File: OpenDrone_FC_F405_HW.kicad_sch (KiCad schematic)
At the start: 83 parts, among them J1 Conn_01x05, J10 Conn_01x02, J11 Conn_01x05, J12 Conn_01x05, J13 Conn_01x02, J14 Conn_01x02, J15 Conn_02x04_Odd_Even, J16 Conn_01x05, J2 Conn_01x02, J3 Conn_01x02, J4 Conn_01x02, J5 Conn_01x02, J6 Conn_01x08, J7 Conn_01x02, J8 Conn_01x04, J9 Conn_01x02, U1 STM32F405RGTx, U2 TPS5430DDA, U3 TPS5430DDA, U4 MPU6000, U5 HMC5883L, U6 BMP280, U8 Board, Y1 8MHz

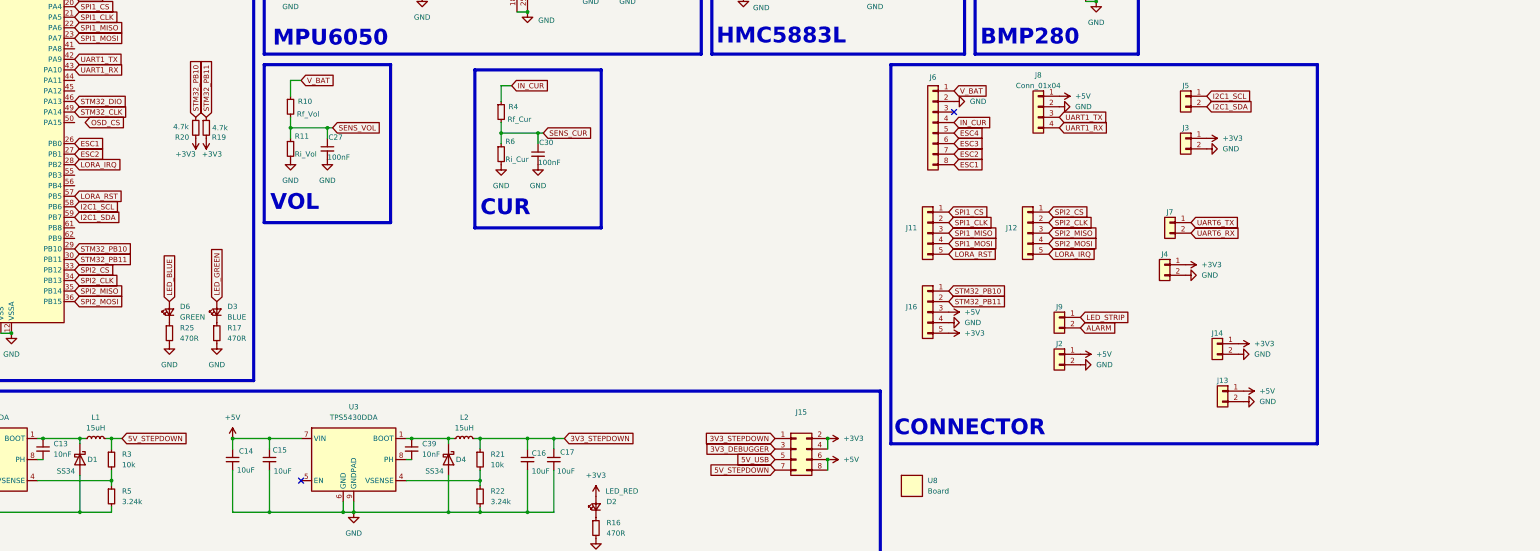
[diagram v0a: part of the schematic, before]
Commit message: update project
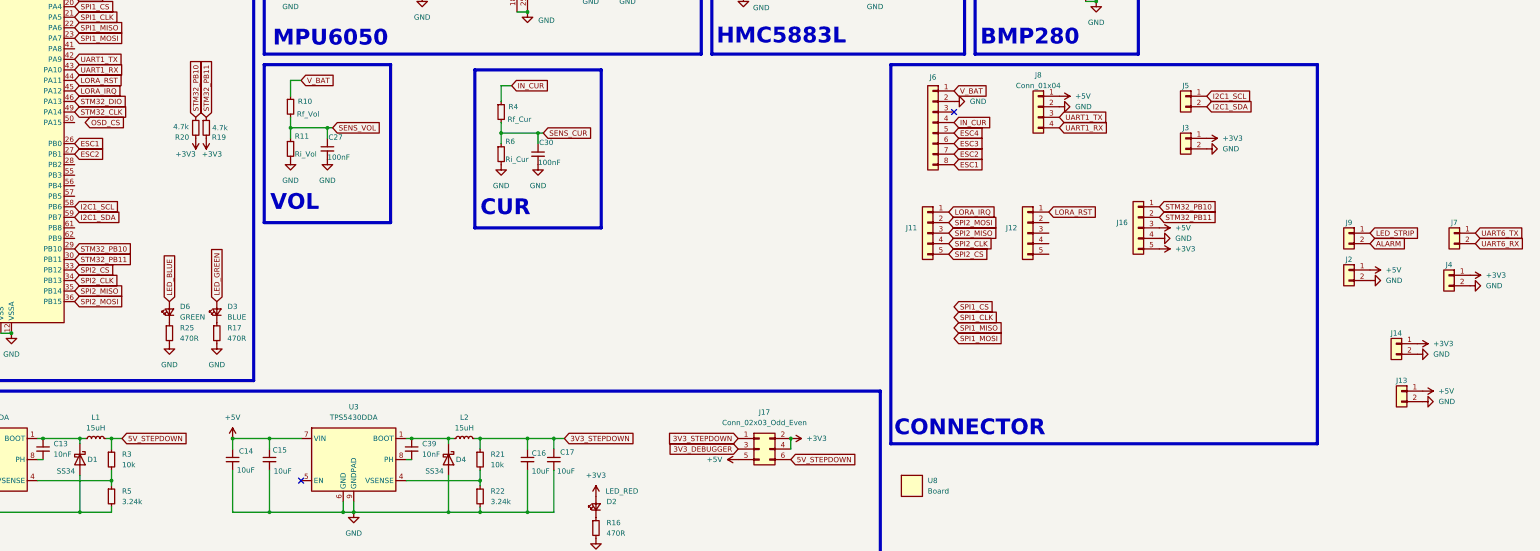
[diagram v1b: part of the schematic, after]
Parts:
- removed J15: Conn_02x04_Odd_Even, Connector_PinHeader_1.27mm:PinHeader_2x04_P1.27mm_Vertical, symbol Connector_Generic:Conn_02x04_Odd_Even
- added J17: Conn_02x03_Odd_Even, Connector_PinHeader_1.27mm:PinHeader_2x03_P1.27mm_Vertical, symbol Connector_Generic:Conn_02x03_Odd_Even
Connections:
- net +3V3: now also J17.2 (Pin_2), J17.4 (Pin_4)
- net +5V: now also J17.5 (Pin_5)
- net 3V3_DEBUGGER: now also J17.3 (Pin_3)
- net 3V3_STEPDOWN: now also J17.1 (Pin_1)
- net 5V_STEPDOWN: now also J17.6 (Pin_6)
- net LORA_IRQ: now also J11.1 (Pin_1), U1.45 (PA12); no longer J12.5 (Pin_5), U1.28 (PB2)
- net LORA_RST: now also J12.1 (Pin_1), U1.44 (PA11); no longer J11.5 (Pin_5), U1.57 (PB5)
- net SPI1_CLK: no longer J11.2 (Pin_2)
- net SPI1_CS: no longer J11.1 (Pin_1)
- net SPI1_MISO: no longer J11.3 (Pin_3)
- net SPI1_MOSI: no longer J11.4 (Pin_4)
- net SPI2_CLK: now also J11.4 (Pin_4); no longer J12.2 (Pin_2)
- net SPI2_CS: now also J11.5 (Pin_5); no longer J12.1 (Pin_1)
- net SPI2_MISO: now also J11.3 (Pin_3); no longer J12.3 (Pin_3)
- net SPI2_MOSI: now also J11.2 (Pin_2); no longer J12.4 (Pin_4)
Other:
- moved on the sheet: J13, J14, J16, J2, J4, J7, J9

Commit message: update project
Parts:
- removed J10: Conn_01x02, Footprint:MountingPad_Battery, symbol Connector_Generic:Conn_01x02
- removed R19, R20: 4.7k, Resistor_SMD:R_0402_1005Metric, symbol Device:R_Small
- added C34: 100nF, Capacitor_SMD:C_0402_1005Metric, symbol Device:C_Small
- added SW1: RESET, Footprint:Button_SMD_4.2x3.3x2.5mm, symbol Switch:SW_Push
- C15: footprint Capacitor_SMD:C_1210_3225Metric -> Capacitor_SMD:C_1206_3216Metric
- J11, J12, J16: footprint Connector_PinHeader_2.00mm:PinHeader_1x05_P2.00mm_Vertical -> Footprint:Header_1x05_P2.00mm_Vertical
- J17: footprint Connector_PinHeader_1.27mm:PinHeader_2x03_P1.27mm_Vertical -> Connector_PinHeader_2.00mm:PinHeader_2x03_P2.00mm_Vertical
- L1, L2: footprint Footprint:Inductor_SMD_5D28 -> Footprint:Inductor_SMD_4D28
- U6: footprint Package_LGA:Bosch_LGA-8_2x2.5mm_P0.65mm_ClockwisePinNumbering -> Footprint:LGA-8_2x2.5mm_P0.65mm
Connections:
- net +3V3: now also J11.5 (Pin_5); no longer J14.1 (Pin_1), J16.5 (Pin_5), J3.1 (Pin_1), J4.1 (Pin_1)
- net +5V: now also J16.5 (Pin_5), J3.1 (Pin_1), J4.1 (Pin_1); no longer J16.3 (Pin_3)
- net 3V3_DEBUGGER: now also J17.1 (Pin_1); no longer J17.3 (Pin_3)
- net 3V3_STEPDOWN: now also J17.3 (Pin_3); no longer J17.1 (Pin_1)
- net ESC1: now also U1.16 (PA2); no longer U1.26 (PB0)
- net ESC2: now also U1.17 (PA3); no longer U1.27 (PB1)
- net ESC3: now also U1.26 (PB0); no longer U1.17 (PA3)
- net ESC4: now also U1.27 (PB1); no longer U1.16 (PA2)
- net GND: now also J1.2 (Pin_2), J12.5 (Pin_5), C34.2, SW1.1; no longer J1.5 (Pin_5), J14.2 (Pin_2), J16.4 (Pin_4)
- net I2C1_SCL: now also J12.4 (Pin_4); no longer J5.1 (Pin_1), R8.2, U4.23 (SCL/SCLK), U6.4 (SCK)
- net I2C1_SDA: now also J12.3 (Pin_3); no longer J5.2 (Pin_2), R7.2, U4.24 (SDA/SDI), U6.3 (SDI)
- net LED_BLUE: now also U1.40 (PC9); no longer U1.3 (PC14)
- net LED_GREEN: now also U1.39 (PC8); no longer U1.2 (PC13)
- net LORA_IRQ: now also J12.2 (Pin_2); no longer J11.1 (Pin_1)
- net MPU6000_INT: now also U1.11 (PC3); no longer U1.15 (PA1)
- net SPI1_CLK: now also J16.2 (Pin_2)
- net SPI1_CS: now also J16.1 (Pin_1)
- net SPI1_MISO: now also J16.3 (Pin_3)
- net SPI1_MOSI: now also J16.4 (Pin_4)
- net SPI2_CLK: now also J11.3 (Pin_3); no longer J11.4 (Pin_4)
- net SPI2_CS: now also J11.4 (Pin_4); no longer J11.5 (Pin_5)
- net SPI2_MISO: now also J11.2 (Pin_2); no longer J11.3 (Pin_3)
- net SPI2_MOSI: now also J11.1 (Pin_1); no longer J11.2 (Pin_2)
- net STM32_CLK: now also J1.4 (Pin_4); no longer J1.3 (Pin_3)
- net STM32_DIO: now also J1.5 (Pin_5); no longer J1.2 (Pin_2)
- net STM32_NRST: now also J1.3 (Pin_3), C34.1, SW1.2; no longer J1.4 (Pin_4)
- net UART4_TX: now reaches U1.14 (PA0)
- net UART4_TX: now also J14.1 (Pin_1)
- net LED_STRIP2: now reaches U1.61 (PB8)
- net LED_STRIP2: now also J9.2 (Pin_2)
- net LED_STRIP1: now reaches U1.62 (PB9)
- net LED_STRIP1: now also J9.1 (Pin_1)
- net ALARM: no longer names the net of U1.8 (PC0)
- net ALARM: no longer J9.2 (Pin_2)
- net LED_STRIP: no longer names the net of U1.4 (PC15)
- net LED_STRIP: no longer J9.1 (Pin_1)
- net STM32_PB10 renamed I2C2_SCL
- net I2C2_SCL: now also J5.1 (Pin_1), R8.2, U4.23 (SCL/SCLK), U6.4 (SCK); no longer J16.1 (Pin_1)
- net STM32_PB11 renamed I2C2_SDA
- net I2C2_SDA: now also J5.2 (Pin_2), R7.2, U4.24 (SDA/SDI), U6.3 (SDI); no longer J16.2 (Pin_2)
- new net UART4_RX: J14.2 (Pin_2), U1.15 (PA1)
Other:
- moved on the sheet: J14, R1

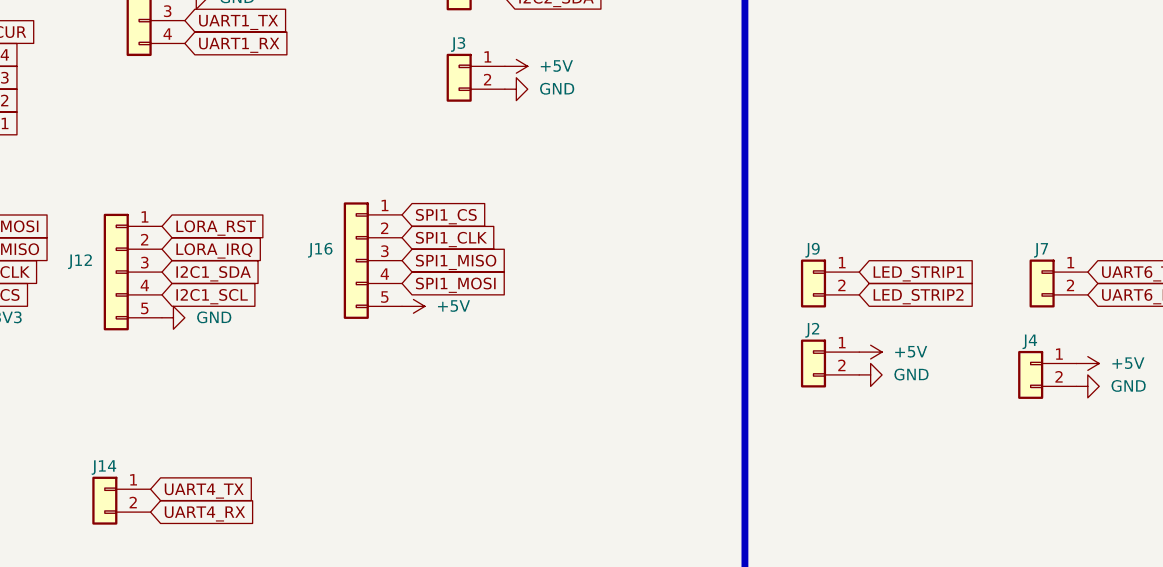
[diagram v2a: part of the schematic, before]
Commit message: update project
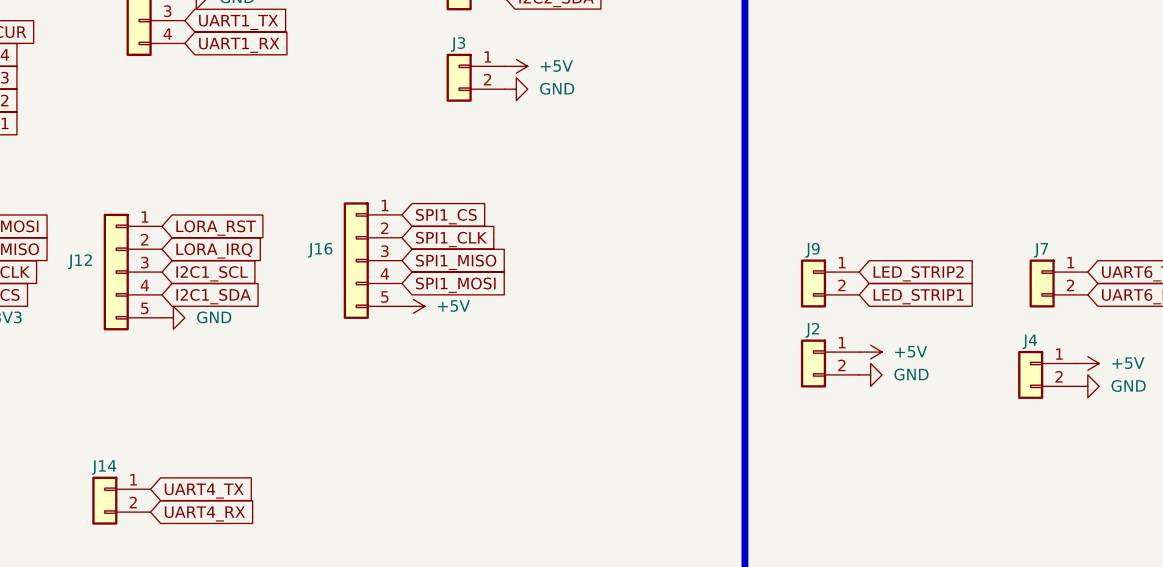
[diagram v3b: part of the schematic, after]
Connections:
- net I2C1_SCL: now also J12.3 (Pin_3); no longer J12.4 (Pin_4)
- net I2C1_SDA: now also J12.4 (Pin_4); no longer J12.3 (Pin_3)
- net LED_STRIP1: now also J9.2 (Pin_2); no longer J9.1 (Pin_1)
- net LED_STRIP2: now also J9.1 (Pin_1); no longer J9.2 (Pin_2)
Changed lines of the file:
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@@
 	(global_label "LED_STRIP1"
 		(shape input)
+		(at 396.24 115.57 0)
+		(fields_autoplaced yes)
+		(effects
+			(font
+				(size 1.27 1.27)
+			)
+			(justify left)
+		)
+		(property "Intersheetrefs" "${INTERSHEET_REFS}"
+			(at 410.1713 115.57 0)
+			(effects
+				(font
+					(size 1.27 1.27)
+				)
+				(justify left)
+				(hide yes)
+			)
+		)
+	)
+	(global_label "I2C1_SDA"
+		(shape input)
+		(at 318.77 115.57 0)
+		(fields_autoplaced yes)
+		(effects
+			(font
+				(size 1.27 1.27)
+			)
+			(justify left)
+		)
+		(property "Intersheetrefs" "${INTERSHEET_REFS}"
+			(at 330.5847 115.57 0)
+			(effects
+				(font
+					(size 1.27 1.27)
+				)
+				(justify left)
+				(hide yes)
+			)
+		)
+	)
+	(global_label "STM32_NRST"
+		(shape input)
+		(at 48.26 48.26 180)
+		(fields_autoplaced yes)
+		(effects
+			(font
+				(size 1.27 1.27)
+			)
+			(justify right)
+		)
+		(property "Intersheetrefs" "${INTERSHEET_REFS}"
+			(at 33.4821 48.26 0)
+			(effects
+				(font
+					(size 1.27 1.27)
+				)
+				(justify right)
+				(hide yes)
+			)
+		)
+	)
+	(global_label "I2C1_SCL"
+		(shape input)
+		(at 318.77 113.03 0)
+		(fields_autoplaced yes)
+		(effects
+			(font
+				(size 1.27 1.27)
+			)
+			(justify left)
+		)
+		(property "Intersheetrefs" "${INTERSHEET_REFS}"
+			(at 330.5242 113.03 0)
+			(effects
+				(font
+					(size 1.27 1.27)
+				)
+				(justify left)
+				(hide yes)
+			)
+		)
+	)
+	(global_label "I2C2_SCL"
+		(shape input)
+		(at 151.13 29.21 180)
+		(fields_autoplaced yes)
+		(effects
+			(font
+				(size 1.27 1.27)
+			)
+			(justify right)
+		)
+		(property "Intersheetrefs" "${INTERSHEET_REFS}"
+			(at 139.3758 29.21 0)
+			(effects
+				(font
+					(size 1.27 1.27)
+				)
+				(justify right)
+				(hide yes)
+			)
+		)
+	)
+	(global_label "UART4_RX"
+		(shape input)
+		(at 83.82 50.8 0)
+		(fields_autoplaced yes)
+		(effects
+			(font
+				(size 1.27 1.27)
+			)
+			(justify left)
+		)
+		(property "Intersheetrefs" "${INTERSHEET_REFS}"
+			(at 96.1185 50.8 0)
+			(effects
+				(font
+					(size 1.27 1.27)
+				)
+				(justify left)
+				(hide yes)
+			)
+		)
+	)
+	(global_label "LED_STRIP2"
+		(shape input)
+		(at 83.82 111.76 0)
+		(fields_autoplaced yes)
+		(effects
+			(font
+				(size 1.27 1.27)
+			)
+			(justify left)
+		)
+		(property "Intersheetrefs" "${INTERSHEET_REFS}"
+			(at 97.7513 111.76 0)
+			(effects
+				(font
+					(size 1.27 1.27)
+				)
+				(justify left)
+				(hide yes)
+			)
+		)
+	)
+	(global_label "5V_STEPDOWN"
+		(shape input)
+		(at 256.54 167.64 0)
+		(fields_autoplaced yes)
+		(effects
+			(font
+				(size 1.27 1.27)
+			)
+			(justify left)
+		)
+		(property "Intersheetrefs" "${INTERSHEET_REFS}"
+			(at 272.7694 167.64 0)
+			(effects
+				(font
+					(size 1.27 1.27)
+				)
+				(justify left)
+				(hide yes)
+			)
+		)
+	)
+	(global_label "IN_CUR"
+		(shape input)
+		(at 189.23 77.47 0)
+		(fields_autoplaced yes)
+		(effects
+			(font
+				(size 1.27 1.27)
+			)
+			(justify left)
+		)
+		(property "Intersheetrefs" "${INTERSHEET_REFS}"
+			(at 198.9886 77.47 0)
+			(effects
+				(font
+					(size 1.27 1.27)
+				)
+				(justify left)
+				(hide yes)
+			)
+		)
+	)
+	(global_label "LED_STRIP2"
+		(shape input)
 		(at 396.24 113.03 0)
 		(fields_autoplaced yes)
@@
 			(effects
 				(font
-					(size 1.27 1.27)
-				)
-				(justify left)
-				(hide yes)
-			)
-		)
-	)
-	(global_label "I2C1_SDA"
-		(shape input)
-		(at 318.77 113.03 0)
-		(fields_autoplaced yes)
-		(effects
-			(font
-				(size 1.27 1.27)
-			)
-			(justify left)
-		)
-		(property "Intersheetrefs" "${INTERSHEET_REFS}"
-			(at 330.5847 113.03 0)
-			(effects
-				(font
-					(size 1.27 1.27)
-				)
-				(justify left)
-				(hide yes)
-			)
-		)
-	)
-	(global_label "STM32_NRST"
-		(shape input)
-		(at 48.26 48.26 180)
-		(fields_autoplaced yes)
-		(effects
-			(font
-				(size 1.27 1.27)
-			)
-			(justify right)
-		)
-		(property "Intersheetrefs" "${INTERSHEET_REFS}"
-			(at 33.4821 48.26 0)
-			(effects
-				(font
-					(size 1.27 1.27)
-				)
-				(justify right)
-				(hide yes)
-			)
-		)
-	)
-	(global_label "I2C1_SCL"
-		(shape input)
-		(at 318.77 115.57 0)
-		(fields_autoplaced yes)
-		(effects
-			(font
-				(size 1.27 1.27)
-			)
-			(justify left)
-		)
-		(property "Intersheetrefs" "${INTERSHEET_REFS}"
-			(at 330.5242 115.57 0)
-			(effects
-				(font
-					(size 1.27 1.27)
-				)
-				(justify left)
-				(hide yes)
-			)
-		)
-	)
-	(global_label "I2C2_SCL"
-		(shape input)
-		(at 151.13 29.21 180)
-		(fields_autoplaced yes)
-		(effects
-			(font
-				(size 1.27 1.27)
-			)
-			(justify right)
-		)
-		(property "Intersheetrefs" "${INTERSHEET_REFS}"
-			(at 139.3758 29.21 0)
-			(effects
-				(font
-					(size 1.27 1.27)
-				)
-				(justify right)
-				(hide yes)
-			)
-		)
-	)
-	(global_label "UART4_RX"
-		(shape input)
-		(at 83.82 50.8 0)
-		(fields_autoplaced yes)
-		(effects
-			(font
-				(size 1.27 1.27)
-			)
-			(justify left)
-		)
-		(property "Intersheetrefs" "${INTERSHEET_REFS}"
-			(at 96.1185 50.8 0)
-			(effects
-				(font
-					(size 1.27 1.27)
-				)
-				(justify left)
-				(hide yes)
-			)
-		)
-	)
-	(global_label "LED_STRIP2"
-		(shape input)
-		(at 83.82 111.76 0)
-		(fields_autoplaced yes)
-		(effects
-			(font
-				(size 1.27 1.27)
-			)
-			(justify left)
-		)
-		(property "Intersheetrefs" "${INTERSHEET_REFS}"
-			(at 97.7513 111.76 0)
-			(effects
-				(font
-					(size 1.27 1.27)
-				)
-				(justify left)
-				(hide yes)
-			)
-		)
-	)
-	(global_label "5V_STEPDOWN"
-		(shape input)
-		(at 256.54 167.64 0)
-		(fields_autoplaced yes)
-		(effects
-			(font
-				(size 1.27 1.27)
-			)
-			(justify left)
-		)
-		(property "Intersheetrefs" "${INTERSHEET_REFS}"
-			(at 272.7694 167.64 0)
-			(effects
-				(font
-					(size 1.27 1.27)
-				)
-				(justify left)
-				(hide yes)
-			)
-		)
-	)
-	(global_label "IN_CUR"
-		(shape input)
-		(at 189.23 77.47 0)
-		(fields_autoplaced yes)
-		(effects
-			(font
-				(size 1.27 1.27)
-			)
-			(justify left)
-		)
-		(property "Intersheetrefs" "${INTERSHEET_REFS}"
-			(at 198.9886 77.47 0)
-			(effects
-				(font
-					(size 1.27 1.27)
-				)
-				(justify left)
-				(hide yes)
-			)
-		)
-	)
-	(global_label "LED_STRIP2"
-		(shape input)
-		(at 396.24 115.57 0)
-		(fields_autoplaced yes)
-		(effects
-			(font
-				(size 1.27 1.27)
-			)
-			(justify left)
-		)
-		(property "Intersheetrefs" "${INTERSHEET_REFS}"
-			(at 410.1713 115.57 0)
-			(effects
-				(font

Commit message: update project
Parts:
- removed Y1: 8MHz, Crystal:Crystal_SMD_3225-4Pin_3.2x2.5mm, symbol Device:Crystal_Small
- added Y2: 8Mhz, Crystal:Crystal_SMD_3225-4Pin_3.2x2.5mm, symbol Device:Crystal_GND24_Small
- D2: value LED_RED -> RED
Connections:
- net GND: now also Y2.2, Y2.4
- net at C9.2, U1.5 (PH0): now also Y2.3
- net at C10.2, U1.6 (PH1): now also Y2.1
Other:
- note added: "CUR SENS"
- note added: "LED"
- note added: "VOL SENS"
- note removed: "CUR"
- note removed: "VOL"
- moved on the sheet: C1, C10, C18, C19, C2, C20, C21, C22, C23, C24, C25, C26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
